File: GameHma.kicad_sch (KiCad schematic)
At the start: 14 parts, among them J1 Screw_Terminal_01x02, J2 Motor_Terminal_01x04, J3 Motor_Terminal_01x04, J4 Motor_Terminal_01x04, J5 Motor_Terminal_01x04, U1 ESP32-DEVKIT-V1, U2 A4988_STEPPER_MOTOR_DRIVER_CA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, U3 A4988_STEPPER_MOTOR_DRIVER_CA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, U4 A4988_STEPPER_MOTOR_DRIVER_CA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, U5 A4988_STEPPER_MOTOR_DRIVER_CA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

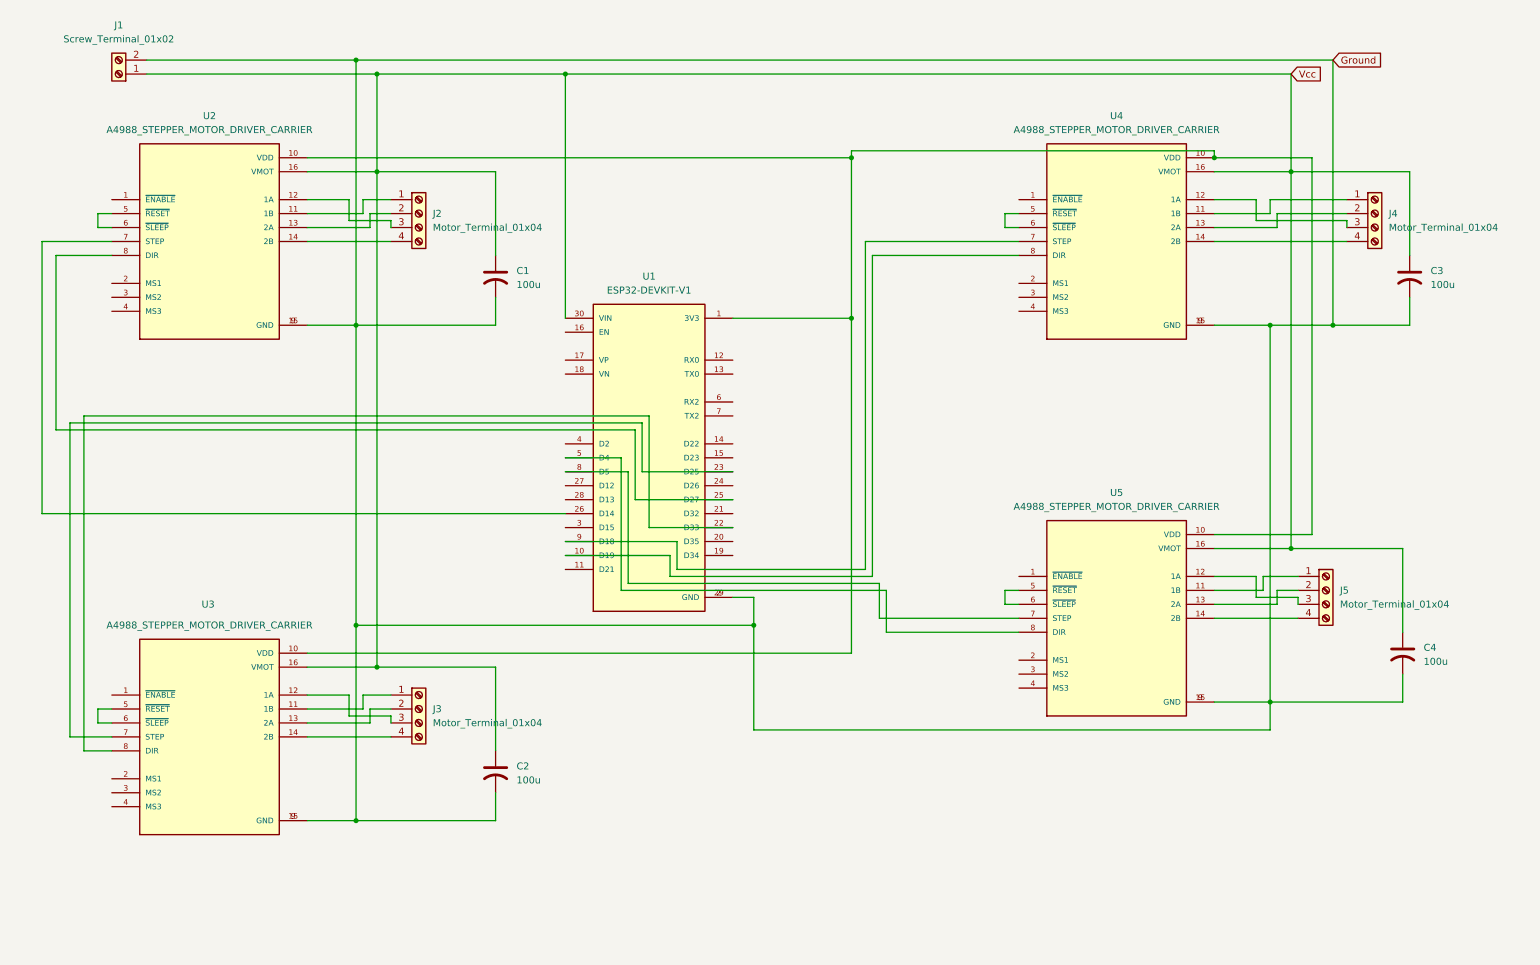
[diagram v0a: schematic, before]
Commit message: example of how it's done done done
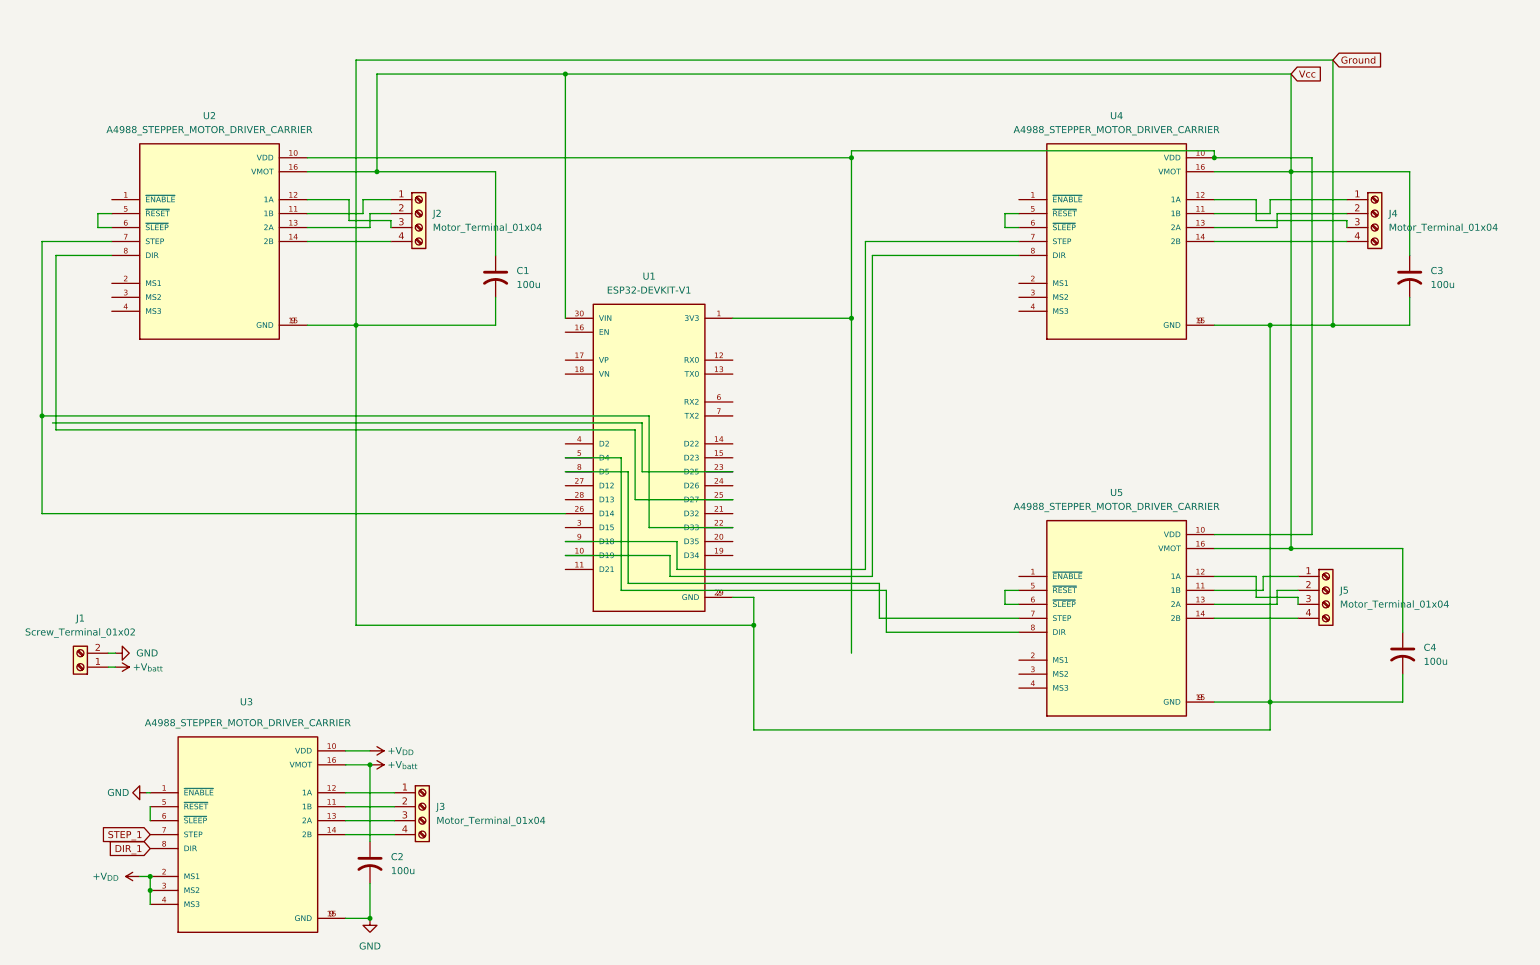
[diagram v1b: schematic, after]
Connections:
- net Ground: no longer C2.2, J1.2 (Pin_2), U3.15 (GND), U3.9 (GND)
- net Vcc: no longer C2.1, J1.1 (Pin_1), U3.16 (VMOT)
- net at U1.1 (3V3), U2.10 (VDD), U4.10 (VDD)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: no longer U3.10 (VDD)
- net at U1.26 (D14), U2.7 (STEP): now also U1.22 (D33)
- net GND: now reaches U3.1 (~{ENABLE})
- net GND: now also C2.2, J1.2 (Pin_2), U3.15 (GND), U3.9 (GND)
- net at U3.11 (1B): now also J3.2 (Pin_2); no longer J3.1 (Pin_1)
- net at U3.12 (1A): now also J3.1 (Pin_1); no longer J3.3 (Pin_3)
- net at U3.13 (2A): now also J3.3 (Pin_3); no longer J3.2 (Pin_2)
- net +V_{DD}: now reaches U3.2 (MS1)
- net +V_{DD}: now also U3.10 (VDD), U3.3 (MS2), U3.4 (MS3)
- net at U1.23 (D25): no longer U3.7 (STEP)
- net DIR_1: now reaches U3.8 (DIR)
- net DIR_1: no longer U1.22 (D33)
- new net +V_{batt}: C2.1, J1.1 (Pin_1), U3.16 (VMOT)
- new net STEP_1: U3.7 (STEP)
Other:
- moved on the sheet: C2, J1, J3, U3

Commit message: nothing
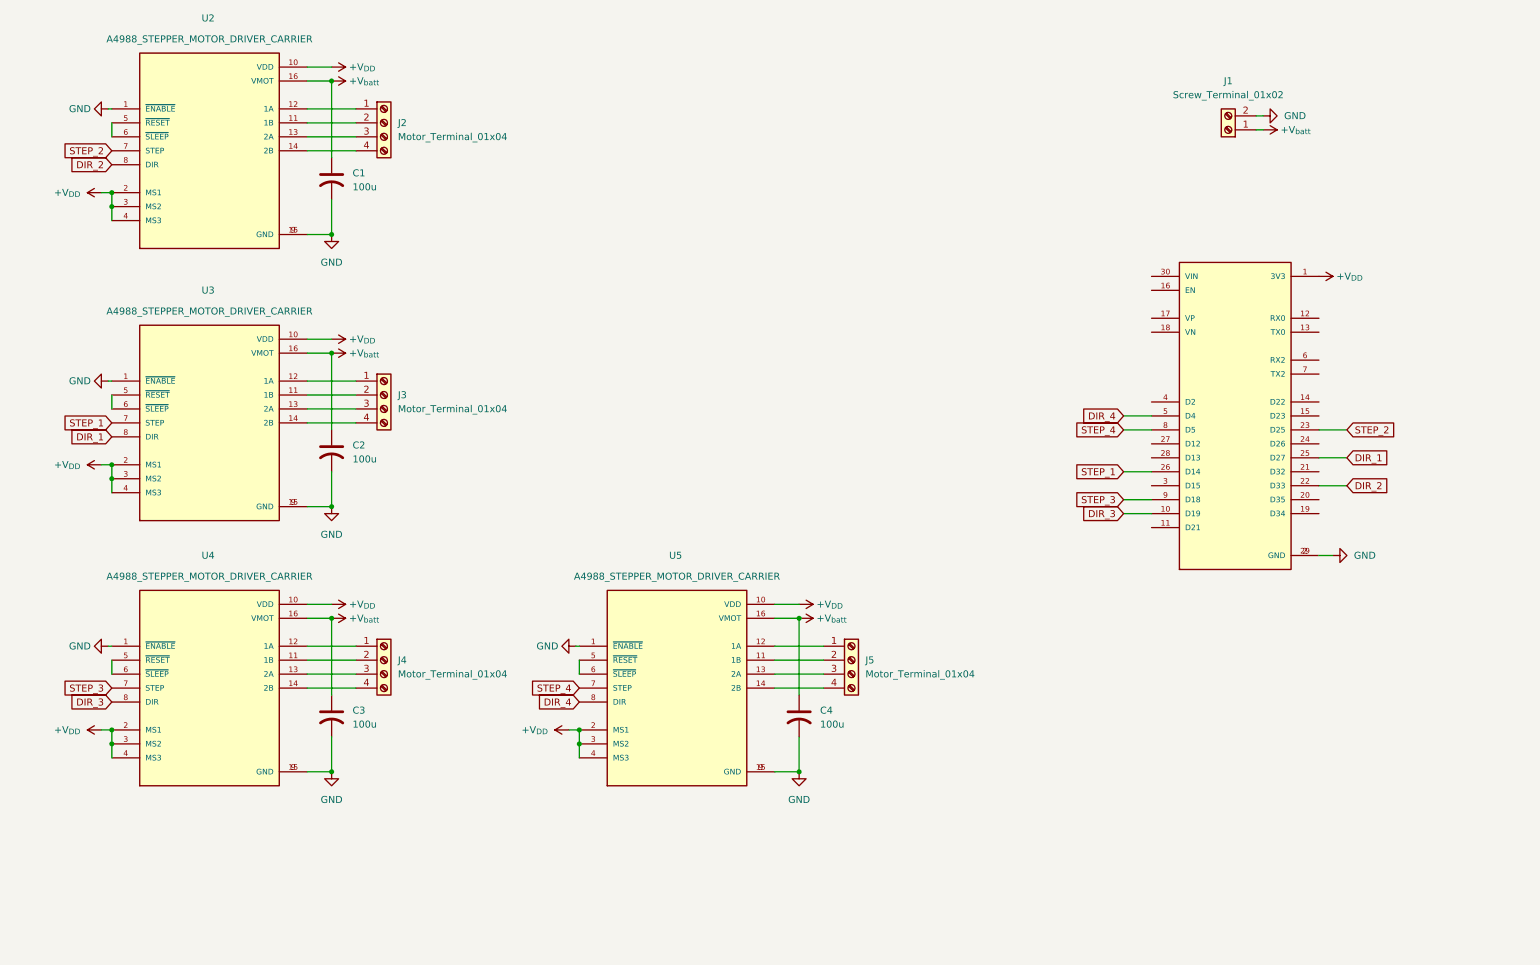
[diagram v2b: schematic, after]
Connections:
- net Ground is gone; now on net GND: C1.2, C3.2, C4.2, U1.2 (GND), U1.29 (GND), U2.15 (GND), U2.9 (GND), U4.15 (GND), U4.9 (GND), U5.15 (GND), U5.9 (GND)
- net +V_{DD}: now also U1.1 (3V3), U2.10 (VDD), U2.2 (MS1), U2.3 (MS2), U2.4 (MS3), U4.10 (VDD), U4.2 (MS1), U4.3 (MS2), U4.4 (MS3), U5.10 (VDD), U5.2 (MS1), U5.3 (MS2), U5.4 (MS3)
- net +V_{batt}: now also C1.1, C3.1, C4.1, U2.16 (VMOT), U4.16 (VMOT), U5.16 (VMOT)
- net DIR_1: now also U1.25 (D27)
- net GND: now also U2.1 (~{ENABLE}), U4.1 (~{ENABLE}), U5.1 (~{ENABLE})
- net STEP_1: now also U1.26 (D14)
- net at U2.11 (1B): now also J2.2 (Pin_2); no longer J2.1 (Pin_1)
- net at U2.13 (2A): now also J2.3 (Pin_3); no longer J2.2 (Pin_2)
- net at U2.12 (1A): now also J2.1 (Pin_1); no longer J2.3 (Pin_3)
- net DIR_2: now reaches U2.8 (DIR)
- net DIR_2: now also U1.22 (D33); no longer U1.25 (D27)
- net at J5.1 (Pin_1): now also U5.12 (1A); no longer U5.11 (1B)
- net at J5.3 (Pin_3): now also U5.13 (2A); no longer U5.12 (1A)
- net at J5.2 (Pin_2): now also U5.11 (1B); no longer U5.13 (2A)
- net STEP_4: now reaches U1.8 (D5), U5.7 (STEP)
- net DIR_4: now reaches U1.5 (D4), U5.8 (DIR)
- net DIR_3: now reaches U1.10 (D19), U4.8 (DIR)
- net STEP_2: now reaches U1.23 (D25)
- net STEP_2: now also U2.7 (STEP)
- net STEP_3: now reaches U1.9 (D18), U4.7 (STEP)
- net at J4.1 (Pin_1): now also U4.12 (1A); no longer U4.11 (1B)
- net at J4.2 (Pin_2): now also U4.11 (1B); no longer U4.13 (2A)
- net at J4.3 (Pin_3): now also U4.13 (2A); no longer U4.12 (1A)
- removed net Vcc: C1.1, C3.1, C4.1, U1.30 (VIN), U2.16 (VMOT), U4.16 (VMOT), U5.16 (VMOT)
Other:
- moved on the sheet: C2, J1, J3, U3
